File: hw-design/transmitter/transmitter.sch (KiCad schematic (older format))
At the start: 43 parts, among them P1 CONN_01X03, P10 test-double, P11 test-double, P12 OptionC, P2 test-double, P3 test-double, P4 test-double, P5 test-double, P6 CONN_01X02, P7 test-double, P8 OptionB, P9 OptionA, Q1 2N3904, Q2 2N3904, SW1 power, U1 usb-micro, U2 MCP73833, U3 CD4047, U4 CD4047

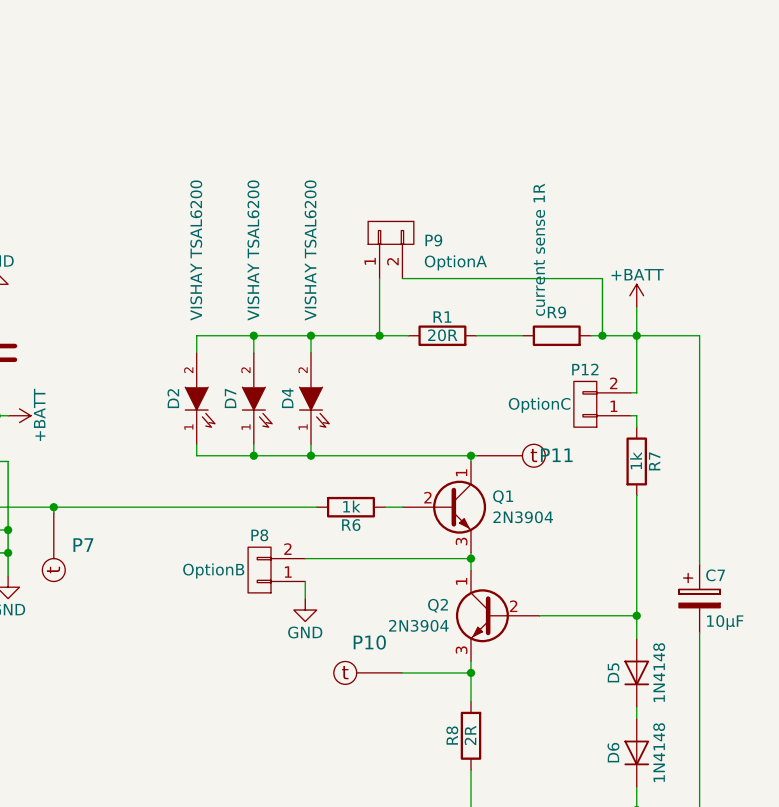
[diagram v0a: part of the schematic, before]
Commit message: Somoe old fixes
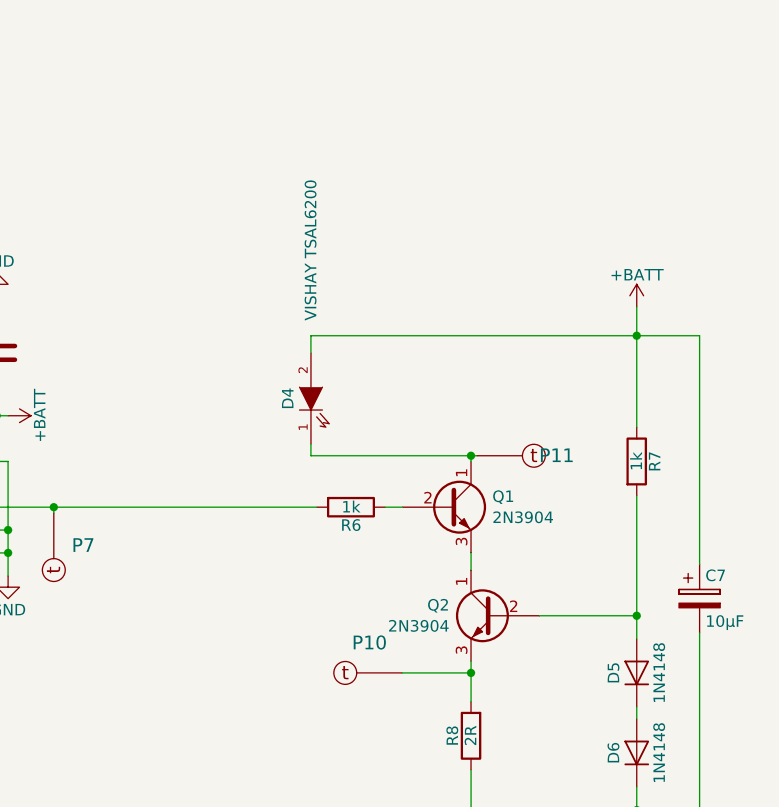
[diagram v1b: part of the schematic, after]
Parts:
- removed D2, D7: VISHAY TSAL6200, LEDs:LED-5MM, symbol LED-RESCUE-transmitter
- removed P12: OptionC, w_pin_strip:pin_socket_2, symbol CONN_01X02
- removed P8: OptionB, w_pin_strip:pin_socket_2, symbol CONN_01X02
- removed P9: OptionA, w_pin_strip:pin_socket_2, symbol CONN_01X02
- removed R1: 20R, w_smd_resistors:r_1210, symbol R
- removed R9: current sense 1R, resistor:0207%2f10, symbol R
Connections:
- net +BATT: now also D4.2 (A), R7.1
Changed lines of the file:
@@
-EESchema Schematic File Version 2
+EESchema Schematic File Version 3
 LIBS:transmitter-rescue
 LIBS:iwasz-kicad
 LIBS:power
 LIBS:device
-LIBS:transistors
-LIBS:conn
 LIBS:linear
 LIBS:regul
-LIBS:74xx
-LIBS:cmos4000
 LIBS:adc-dac
 LIBS:memory
@@
 LIBS:digital-audio
 LIBS:philips
-LIBS:display
 LIBS:cypress
 LIBS:siliconi
@@
 LIBS:atmel
 LIBS:contrib
-LIBS:valves
 LIBS:transmitter-cache
 EELAYER 26 0
@@
 $EndComp
 $Comp
-L LED-RESCUE-transmitter D7
-U 1 1 5643D200
-P 8700 3475
-F 0 "D7" H 8700 3575 50  0000 C CNN
-F 1 "VISHAY TSAL6200" H 9350 3475 50  0000 C CNN
-F 2 "LEDs:LED-5MM" H 8700 3475 60  0001 C CNN
-F 3 "http://pl.farnell.com/vishay/tsal6200/ir-emitter-940nm-5mm-through-hole/dp/3152856?CMP=i-ddd7-00001003" H 8700 3475 60  0001 C CNN
-	1    8700 3475
-	0    -1   -1   0
-$EndComp
-$Comp
 L C C5
 U 1 1 56441557
@@
 	0    1    1    0
 $EndComp
-$Comp
-L R R9
-U 1 1 5684A214
-P 10025 3200
-F 0 "R9" V 10125 3200 50  0000 C CNN
-F 1 "current sense 1R" H 10400 3275 50  0000 C CNN
-F 2 "resistor:0207%2f10" V 9955 3200 50  0001 C CNN
-F 3 "" H 10025 3200 50  0000 C CNN
-	1    10025 3200
-	0    -1   -1   0
-$EndComp
 Wire Wire Line
 	1625 1125 3250 1125
@@
 	9650 5100 9650 5275
 Wire Wire Line
-	8700 3275 8700 3200
-Wire Wire Line
-	8450 3725 9675 3725
-Wire Wire Line
 	4250 3025 4250 3125
 Wire Wire Line
@@
 Connection ~ 4500 3950
 Wire Wire Line
-	10175 3200 10650 3200
+	8950 3200 10650 3200
 $Comp
 L CONN_01X02 P6
@@
 	5375 4125 5625 4125
 Connection ~ 5625 4125
-$Comp
-L LED-RESCUE-transmitter D2
-U 1 1 5685F9CD
-P 8450 3475
-F 0 "D2" H 8450 3575 50  0000 C CNN
-F 1 "VISHAY TSAL6200" H 9100 3475 50  0000 C CNN
-F 2 "LEDs:LED-5MM" H 8450 3475 60  0001 C CNN
-F 3 "http://pl.farnell.com/vishay/tsal6200/ir-emitter-940nm-5mm-through-hole/dp/3152856?CMP=i-ddd7-00001003" H 8450 3475 60  0001 C CNN
-	1    8450 3475
-	0    -1   -1   0
-$EndComp
-Wire Wire Line
-	8450 3275 8450 3200
-$Comp
-L R R1
-U 1 1 56830A1A
-P 9525 3200
-F 0 "R1" V 9605 3200 50  0000 C CNN
-F 1 "20R" V 9525 3200 50  0000 C CNN
-F 2 "w_smd_resistors:r_1210" V 9455 3200 30  0001 C CNN
-F 3 "" H 9525 3200 30  0000 C CNN
-	1    9525 3200
-	0    -1   -1   0
-$EndComp
-Wire Wire Line
-	8450 3725 8450 3675
-Connection ~ 8700 3200
-Connection ~ 8950 3200
-Wire Wire Line
-	8700 3675 8700 3725
-Connection ~ 8700 3725
 Wire Wire Line
 	8950 3675 8950 3725
-Connection ~ 8950 3725
-Wire Wire Line
-	8450 3200 9375 3200
-Wire Wire Line
-	9675 3200 9875 3200
-$Comp
-L CONN_01X02 P9
-U 1 1 568368B3
-P 9300 2750
-F 0 "P9" V 9265 2606 50  0000 R CNN
-F 1 "OptionA" V 9173 2606 50  0000 R CNN
-F 2 "w_pin_strip:pin_socket_2" H 9300 2750 50  0001 C CNN
-F 3 "" H 9300 2750 50  0000 C CNN
-	1    9300 2750
-	0    -1   -1   0
-$EndComp
-Wire Wire Line
-	9250 2950 9250 2950
-Wire Wire Line
-	9250 2950 9250 3200
-Connection ~ 9250 3200
-Wire Wire Line
-	9350 2950 10225 2950
-Wire Wire Line
-	10225 2950 10225 3200
-Connection ~ 10225 3200
-$Comp
-L CONN_01X02 P8
-U 1 1 5683989A
-P 8725 4225
-F 0 "P8" H 8725 4075 50  0000 C CNN
-F 1 "OptionB" H 8925 4225 50  0000 C CNN
-F 2 "w_pin_strip:pin_socket_2" H 8725 4225 50  0001 C CNN
-F 3 "" H 8725 4225 50  0000 C CNN
-	1    8725 4225
-	-1   0    0    1
-$EndComp
-Wire Wire Line
-	8925 4175 9650 4175
-Connection ~ 9650 4175
-$Comp
-L GND #PWR018
-U 1 1 5683A26C
-P 8925 4350
-F 0 "#PWR018" H 8925 4100 50  0001 C CNN
-F 1 "GND" H 8925 4200 50  0000 C CNN
-F 2 "" H 8925 4350 60  0000 C CNN
-F 3 "" H 8925 4350 60  0000 C CNN
-	1    8925 4350
-	1    0    0    -1
-$EndComp
-Wire Wire Line
-	8925 4275 8925 4350
-$Comp
-L CONN_01X02 P12
-U 1 1 56847E4F
-P 10150 3500
-F 0 "P12" H 10150 3350 50  0000 C CNN
-F 1 "OptionC" H 10350 3500 50  0000 C CNN
-F 2 "w_pin_strip:pin_socket_2" H 10150 3500 50  0001 C CNN
-F 3 "" H 10150 3500 50  0000 C CNN
-	1    10150 3500
-	-1   0    0    1
-$EndComp
-Wire Wire Line
-	10375 3450 10350 3450
-Wire Wire Line
-	10375 3075 10375 3450
-Wire Wire Line
-	10350 3550 10375 3550
-Wire Wire Line
-	10375 3550 10375 3600
+Wire Wire Line
+	10375 3075 10375 3600
 Connection ~ 9650 4675
 Connection ~ 2050 3950
@@
 Text Notes 725  4975 0    60   ~ 0
 Zmierzony pobór prądu to 41mA przy baterii na full (4.15V)
+Wire Wire Line
+	8950 3725 9675 3725
 $EndSCHEMATC

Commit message: Many changes
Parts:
- removed P1: CONN_01X03, w_pin_strip:pin_socket_3, symbol CONN_01X03
- removed P10: test-double, iwasz:testpad-2p, symbol test-double
- removed P6: CONN_01X02, w_pin_strip:pin_socket_2, symbol CONN_01X02
- added BT1: Battery_Cell, iwasz:BLM-BH18650-PC2, symbol Device:Battery_Cell
- added R1: 10k, Resistor_SMD:R_0603_1608Metric, symbol Device:R
- added R10: 4R, Resistor_SMD:R_0805_2012Metric, symbol transmitter-rescue:R-RESCUE-transmitter
- added R11: 0R, Resistor_SMD:R_0603_1608Metric, symbol transmitter-rescue:R-RESCUE-transmitter
- added R9: 8R, Resistor_SMD:R_0805_2012Metric, symbol transmitter-rescue:R-RESCUE-transmitter
- added SW2: SW_SP3T, iwasz:switch-3way-8pins-shorted, symbol Switch:SW_SP3T
- C1, C7: symbol CP -> transmitter-rescue:CP-RESCUE-transmitter
- C2, C3, C4, C5, C6: footprint w_smd_cap:c_0603 -> Capacitor_SMD:C_0603_1608Metric; symbol C -> transmitter-rescue:C-RESCUE-transmitter
- D1: symbol Led_x2-CA -> iwasz-kicad:Led_x2-CA
- D4: footprint LEDs:LED-5MM -> LED_THT:LED_D5.0mm; symbol LED-RESCUE-transmitter -> Device:LED; price (none) -> 0.36
- D5, D6: footprint ref-packages:SOD323 -> Diode_SMD:D_SOD-323; symbol D -> Device:D; price (none) -> 0.27
- P11, P2, P3, P4, P7: symbol test-double -> iwasz-kicad:test-double
- P5: symbol test-double-RESCUE-transmitter -> transmitter-rescue:test-double-RESCUE-transmitter
- Q1: footprint w_to:to92_3_flat -> Package_TO_SOT_THT:TO-92; symbol Q_NPN_CBE -> transmitter-rescue:Q_NPN_CBE-RESCUE-transmitter; Datasheet2 (none) -> http://pl.farnell.com/on-semiconductor/2n3904tar/transistor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; price1 (none) -> 0.75; price2 (none) -> 0.36
- Q2: footprint w_to:to92_3_flat -> Package_TO_SOT_THT:TO-92; symbol Q_NPN_CBE -> transmitter-rescue:Q_NPN_CBE-RESCUE-transmitter; Datasheet2 (none) -> http://pl.farnell.com/on-semiconductor/2n3904tar/transistor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; price (none) -> 0.75; price2 (none) -> 0.36
- R2, R3, R4, R5, R6, R7: footprint w_smd_resistors:r_0603 -> Resistor_SMD:R_0603_1608Metric; symbol R -> transmitter-rescue:R-RESCUE-transmitter
- R8: footprint w_smd_resistors:r_1210 -> Resistor_SMD:R_0805_2012Metric; symbol R -> transmitter-rescue:R-RESCUE-transmitter
- RV1, RV2: footprint Potentiometers:Potentiometer_Bourns_3006P_Angular_ScrewFront -> Potentiometer_THT:Potentiometer_Bourns_3296W_Vertical; symbol POT-RESCUE-transmitter -> transmitter-rescue:POT-RESCUE-transmitter
- SW1: footprint w_pin_strip:pin_socket_2 -> Button_Switch_THT:SW_CuK_OS102011MA1QN1_SPDT_Angled; symbol SPST -> Switch:SW_SPDT
- U1: footprint w_conn_pc:conn_usb_B_micro_smd-2 -> iwasz:conn_usb_B_micro_smd-2-nohole; symbol usb-micro -> iwasz-kicad:usb-micro
- U2: footprint ref-packages:MSOP10 -> Package_SSOP:MSOP-10_3x3mm_P0.5mm; symbol MCP73833 -> iwasz-kicad:MCP73833
- U3, U4: footprint Housings_SOIC:SOIC-14_3.9x8.7mm_Pitch1.27mm -> Package_SOIC:SOIC-14_3.9x8.7mm_P1.27mm; symbol CD4047 -> iwasz-kicad:CD4047
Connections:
- net +BATT: now also SW1.1 (A); no longer SW1.2
- net GND: now also BT1.2 (-), R1.1, R10.1, R9.1
- net at U2.10 (VBAT), U2.9 (VBAT): now also SW1.2 (B), BT1.1 (+); no longer SW1.1
- net at U2.8 (THERM): now also R1.2
- net at C2.2, U3.3 (R-C_COM): now also R11.2; no longer RV1.1, RV1.2
- net at Q2.3 (E): now also SW2.3; no longer R8.2
- new net: R11.1, RV1.1, RV1.2
- new net: R8.2, SW2.1
- new net: R10.2, SW2.2
- new net: R9.2, SW2.4
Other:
- note added: "300mA, 2kR = 500mA, 1k2 = 800mA"
- note added: "Dobrać eksperymentalnie.\nOryginalnie był tylko 2R."
- note added: "R11 można wybrać tak, żeby potencjometr\ndziałał jako fine-tune"
- note removed: "300mA, 2kR = 500mA"
- moved on the sheet: R8

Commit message: New version of the transmitter and its enclosure is done
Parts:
- BT1: footprint iwasz:BLM-BH18650-PC2 -> Battery:BatteryHolder_MPD_BH-18650-PC2
- D4: footprint LED_THT:LED_D5.0mm -> LED_THT:LED_D5.0mm_Horizontal_O3.81mm_Z3.0mm
- SW1: footprint Button_Switch_THT:SW_CuK_OS102011MA1QN1_SPDT_Angled -> iwasz:MFP 201 NR
- SW2: footprint iwasz:switch-3way-8pins-shorted -> iwasz:MFP-1323-R
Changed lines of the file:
@@
 F 0 "SW1" H 5225 825 50  0000 C CNN
 F 1 "power" H 5225 900 50  0000 C CNN
-F 2 "Button_Switch_THT:SW_CuK_OS102011MA1QN1_SPDT_Angled" H 5225 725 60  0001 C CNN
+F 2 "iwasz:MFP 201 NR" H 5225 725 60  0001 C CNN
 F 3 "http://lispol.pl/product,2183,wylacznik_kolyskowy_mini_czarny.html" H 5225 725 60  0001 C CNN
 F 4 "Kołyskowy włącznik zasilania." H 5225 725 60  0001 C CNN "Opis"
@@
 F 0 "D4" H 8950 3575 50  0000 C CNN
 F 1 "VISHAY TSAL6200" H 9600 3475 50  0000 C CNN
-F 2 "LED_THT:LED_D5.0mm" H 8950 3475 60  0001 C CNN
+F 2 "LED_THT:LED_D5.0mm_Horizontal_O3.81mm_Z3.0mm" H 8950 3475 60  0001 C CNN
 F 3 "http://pl.farnell.com/vishay/tsal6200/ir-emitter-940nm-5mm-through-hole/dp/3152856?CMP=i-ddd7-00001003" H 8950 3475 60  0001 C CNN
 F 4 "0.36" H 8950 3475 50  0001 C CNN "price"
@@
 F 0 "BT1" V 5530 1175 50  0000 C CNN
 F 1 "Battery_Cell" V 5439 1175 50  0000 C CNN
-F 2 "iwasz:BLM-BH18650-PC2" V 5275 1185 50  0001 C CNN
+F 2 "Battery:BatteryHolder_MPD_BH-18650-PC2" V 5275 1185 50  0001 C CNN
 F 3 "" V 5275 1185 50  0001 C CNN
 	1    5275 1125
@@
 F 0 "SW2" V 9604 4996 50  0000 L CNN
 F 1 "SW_SP3T" V 9695 4996 50  0000 L CNN
-F 2 "iwasz:switch-3way-8pins-shorted" H 9025 5025 50  0001 C CNN
+F 2 "iwasz:MFP-1323-R" H 9025 5025 50  0001 C CNN
 F 3 "" H 9025 5025 50  0001 C CNN
 	1    9650 4850
